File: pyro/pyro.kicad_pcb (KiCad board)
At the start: 2 copper layers, 34.5 x 32 mm, 15 parts, among them J1 Screw_Terminal_01x02, J2 Screw_Terminal_01x02, J3 Screw_Terminal_01x02, Q1 ISA170230C04LMDS, U1 IRLML6344TRPBF

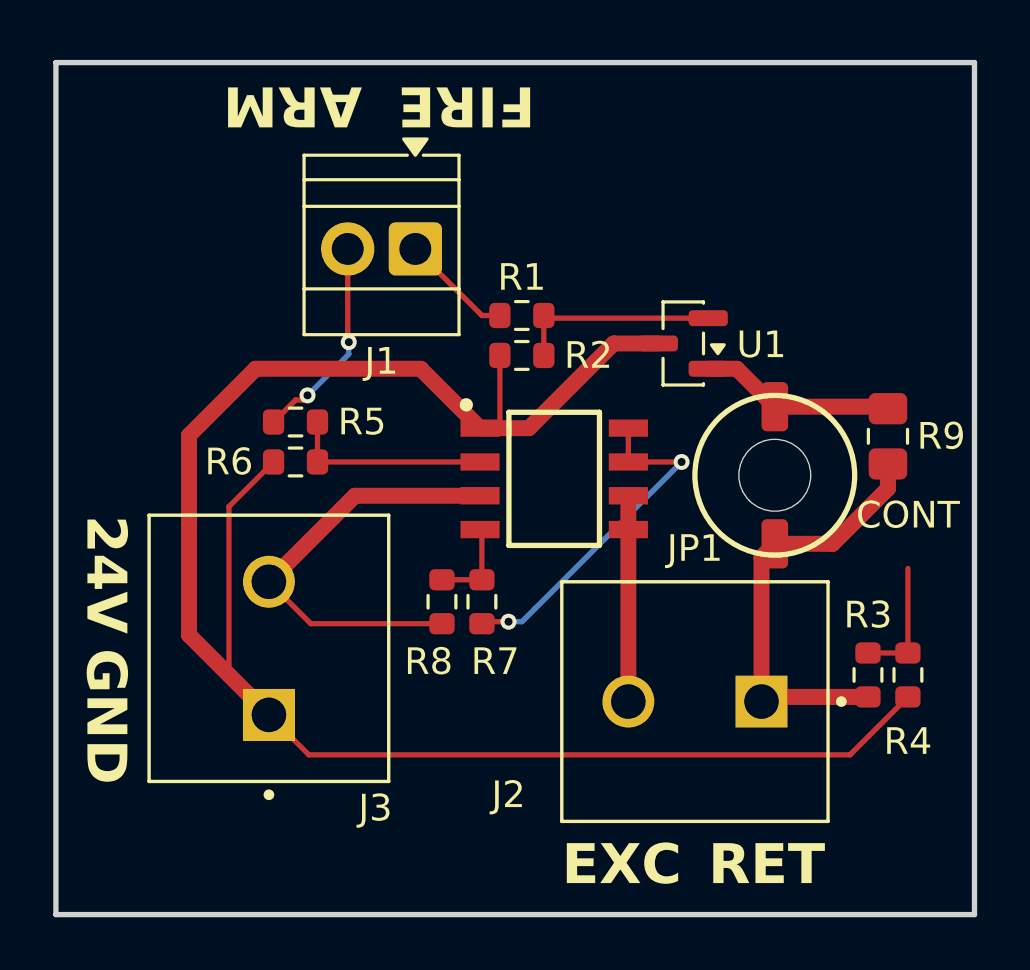
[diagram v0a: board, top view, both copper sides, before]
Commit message: bruh
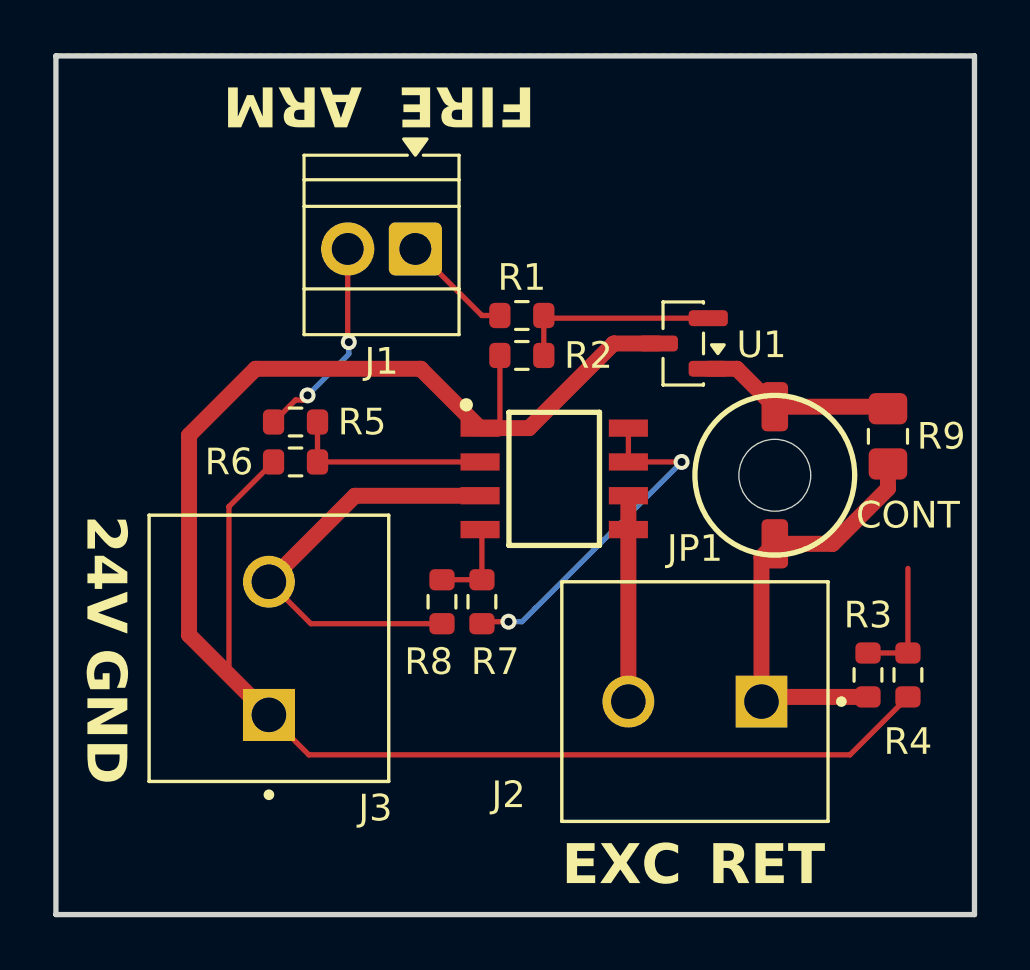
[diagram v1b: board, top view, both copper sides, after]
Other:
- board size 34.5 x 32 mm -> 34.5 x 32.2 mm
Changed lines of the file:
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@@
 	)
 	(gr_rect
-		(start 77 34)
+		(start 77 33.75)
 		(end 111.5 66)
 		(stroke
@@
 		(polygon
 			(pts
-				(xy 77 34) (xy 111.5 34) (xy 111.5 66) (xy 77 66)
-			)
-		)
+				(xy 77 33.690351) (xy 111.5 33.690351) (xy 111.5 66) (xy 77 66)
+			)
+		)
